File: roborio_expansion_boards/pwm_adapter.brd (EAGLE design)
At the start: 16.8 x 76.2 mm, 30 parts

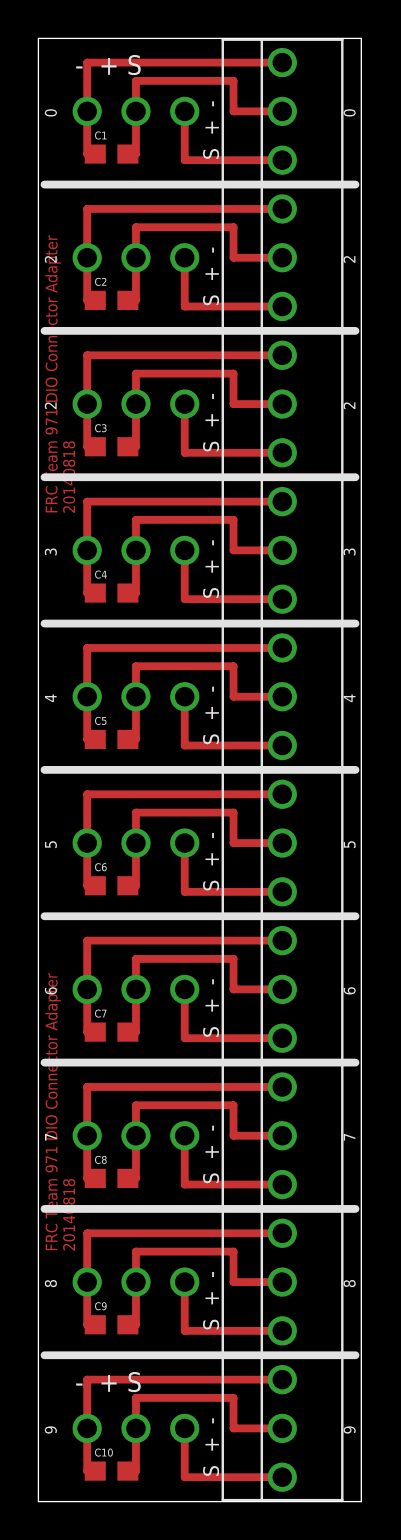
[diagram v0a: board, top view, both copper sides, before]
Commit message: finish PCBs and generate Gerbers for Seeed
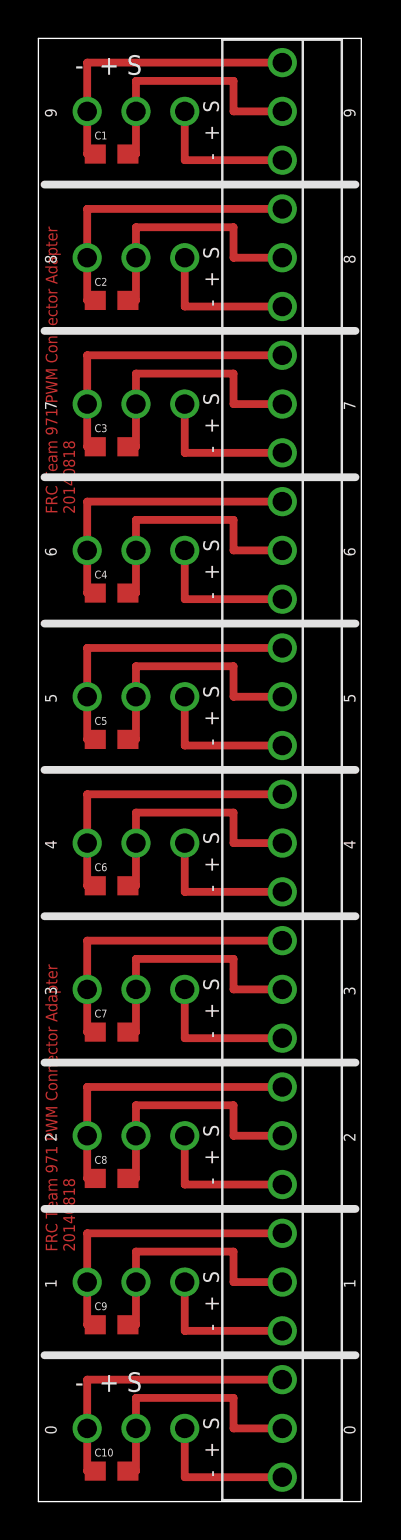
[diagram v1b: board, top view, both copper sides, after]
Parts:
- turned U$11 to 0 degrees
- turned U$12 to 0 degrees
- turned U$13 to 0 degrees
- turned U$14 to 0 degrees
- turned U$15 to 0 degrees
- turned U$16 to 0 degrees
- turned U$17 to 0 degrees
- turned U$18 to 0 degrees
- turned U$19 to 0 degrees
- turned U$20 to 0 degrees
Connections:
- net N$1: now also U$20.1; no longer U$20.3
- net N$10: now also U$13.1; no longer U$13.3
- net N$12: now also U$17.3; no longer U$17.1
- net N$13: now also U$14.1; no longer U$14.3
- net N$15: now also U$16.3; no longer U$16.1
- net N$16: now also U$15.1; no longer U$15.3
- net N$18: now also U$15.3; no longer U$15.1
- net N$19: now also U$16.1; no longer U$16.3
- net N$21: now also U$14.3; no longer U$14.1
- net N$22: now also U$17.1; no longer U$17.3
- net N$24: now also U$13.3; no longer U$13.1
- net N$25: now also U$18.1; no longer U$18.3
- net N$27: now also U$12.3; no longer U$12.1
- net N$28: now also U$19.1; no longer U$19.3
- net N$3: now also U$20.3; no longer U$20.1
- net N$30: now also U$11.3; no longer U$11.1
- net N$4: now also U$11.1; no longer U$11.3
- net N$6: now also U$19.3; no longer U$19.1
- net N$7: now also U$12.1; no longer U$12.3
- net N$9: now also U$18.3; no longer U$18.1
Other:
- board text added: "1"
- board text added: "FRC Team 971 PWM Connector Adapter 20140818"
- board text removed: "FRC Team 971 DIO Connector Adapter 20140818"
- board text removed: "S + -"
